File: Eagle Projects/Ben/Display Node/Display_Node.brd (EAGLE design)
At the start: 100 x 80 mm, 29 parts, among them Q1 16MHz, Q3 16MHz, Q4 16MHz, U1 ATMEGA328P_TQFP, U2 MCP2551

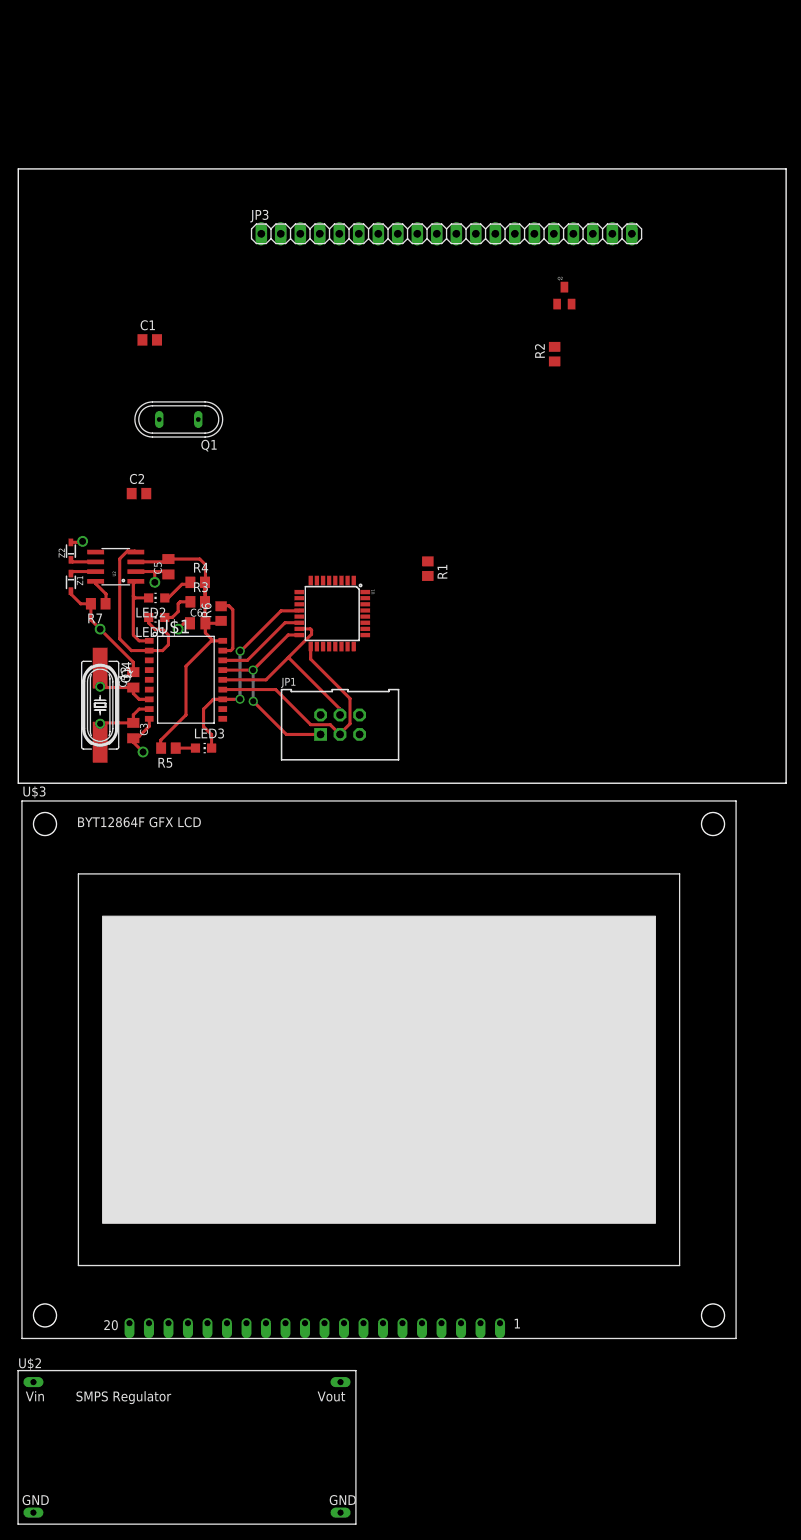
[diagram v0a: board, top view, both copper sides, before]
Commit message: Workin on stuff...
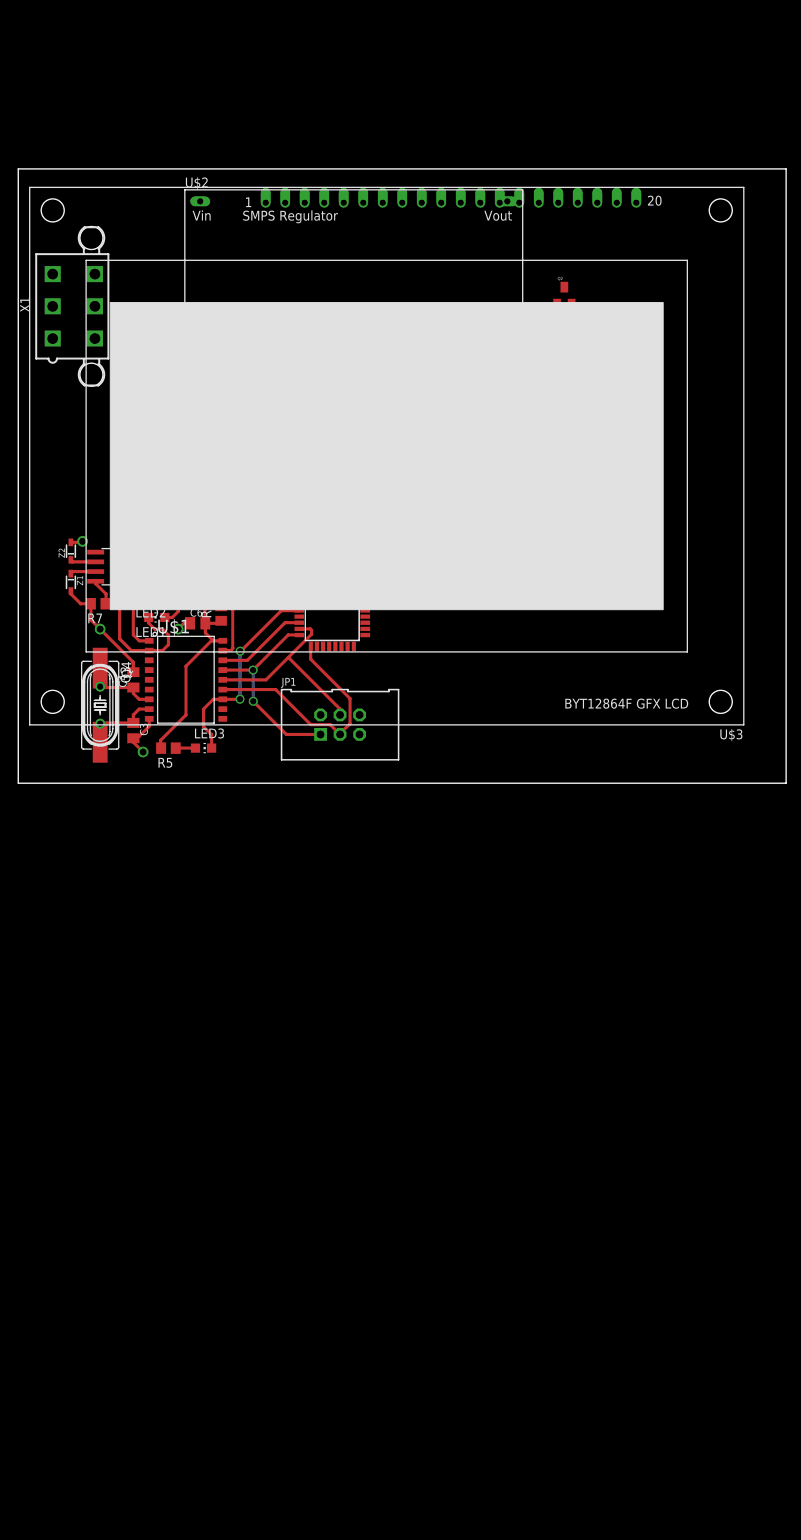
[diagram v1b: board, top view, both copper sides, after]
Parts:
- removed JP3: GFX_LCD, adafruit:1X20
- added X1, X2: 5566-6, con-molex:5566-6
- moved U$3 176.9 mm to (94.5, 77.6), turned to 180 degrees
- moved U$2 155.3 mm to (21.7, 57.3)
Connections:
- new net +12V: U$2.VIN, X1.1, X2.1
- new net LCD_RST: U$3.P$4
- new net N$14: X1.5, X2.5
- new net N$15: X1.6, X2.6
- net +5V: now also U$2.VOUT, U$3.P$19, U$3.P$2; no longer JP3.17, JP3.19, JP3.2
- net CANH: now also X1.3, X2.3
- net CANL: now also X1.4, X2.4
- net GND: now also U$2.GND, U$2.GND@, U$3.P$20, U$3.P$6, X1.2, X2.2; no longer JP3.1, JP3.15
- net LCD_CS: now also U$3.P$17; no longer JP3.4
- net MOSI: now also U$3.P$16; no longer JP3.5
- net N$4: now also U$3.P$1; no longer JP3.20
- net SCK: now also U$3.P$15; no longer JP3.6

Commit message: Almost lost some important stuff! managed to save it :D
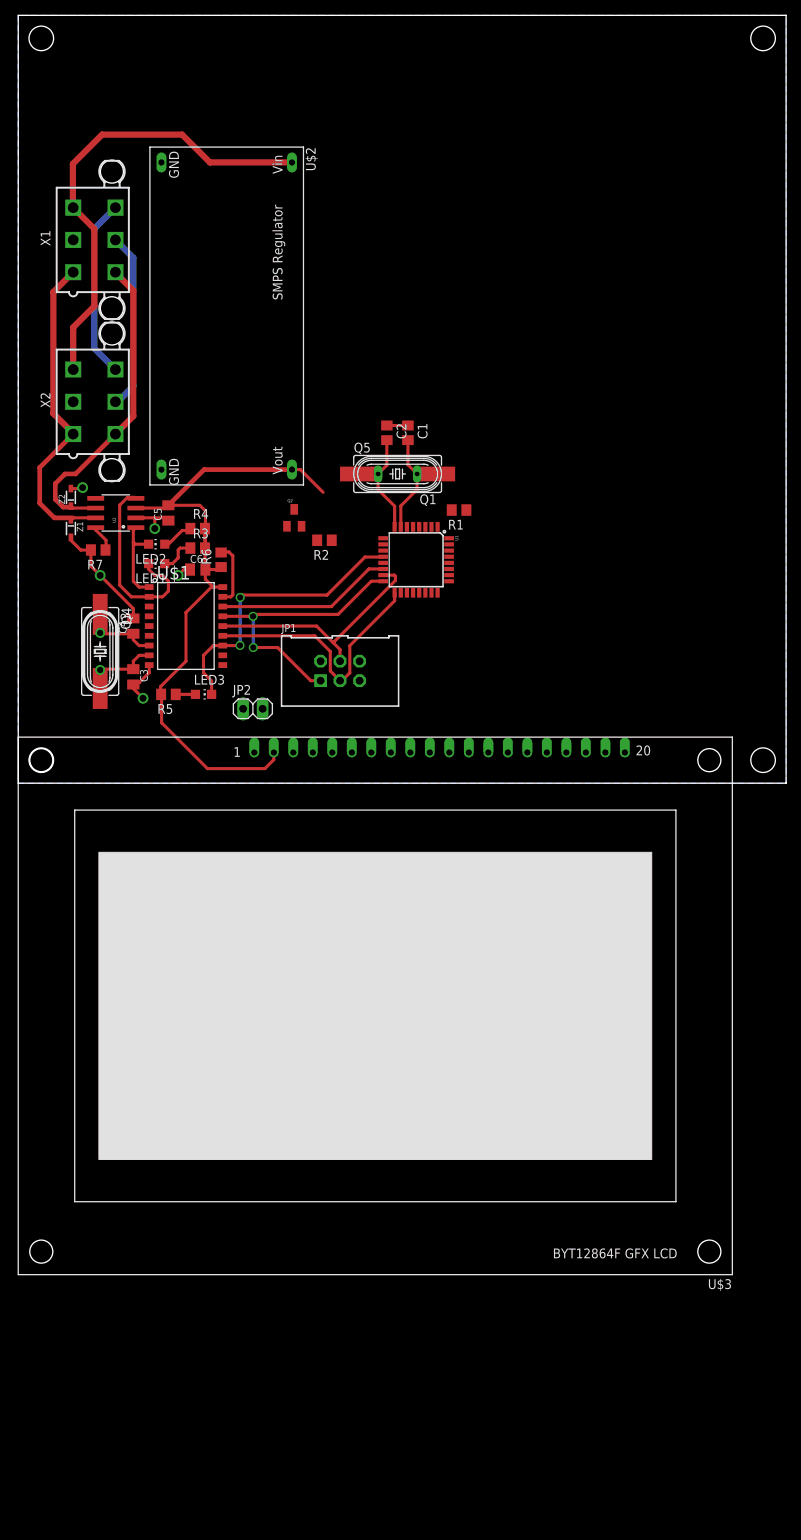
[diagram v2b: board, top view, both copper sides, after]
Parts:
- added JP2: (no value), pinhead:1X02
- added Q5: 16MHz, crystal:HC49UP
- moved U$3 71.6 mm to (93.0, 6.00)
- moved Q2 45.6 mm to (35.9, 34.6)
- moved R2 38.5 mm to (39.9, 31.6), turned to 180 degrees
- moved C1 35.7 mm to (50.7, 45.6), turned to 270 degrees
- moved C2 33.2 mm to (48.0, 45.6), turned to 270 degrees
- moved X2 32.4 mm to (9.91, 49.7)
- moved Q1 29.4 mm to (49.4, 40.3)
- moved U$2 26.0 mm to (17.1, 82.8), turned to 270 degrees
- moved U1 13.0 mm to (51.8, 29.1)
- moved X1 9.05 mm to (9.91, 70.8)
- moved R1 8.65 mm to (57.4, 35.6), turned to 180 degrees
- moved C5 7.00 mm to (19.6, 35.2)
- moved U2 7.00 mm to (12.7, 35.2)
- moved C3 7.00 mm to (15.0, 13.9)
- moved C4 7.00 mm to (15.0, 20.5)
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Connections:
- new net N$10: JP1.2, JP2.2
- net +12V: now also X1.3, X2.3; no longer X1.1, X2.1
- net +5V: now also JP2.1; no longer JP1.2
- net CANH: now also X1.1, X2.1; no longer X1.3, X2.3
- net N$1: now also Q5.2
- net N$2: now also Q5.1
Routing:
- net +12V: track 0.00 -> 60.7 mm
- net +5V: track 44.2 -> 90.3 mm
- net CANH: track 3.33 -> 42.5 mm
- net CANL: track 3.33 -> 41.4 mm
- net N$15: track 0.00 -> 23.4 mm
- net N$14: track 0.00 -> 23.2 mm
- net N$1: track 0.00 -> 12.7 mm
- net N$2: track 0.00 -> 12.7 mm
- net MISO: track 26.5 -> 37.6 mm
- net CANCS: track 12.0 -> 22.9 mm
- net CANINT: track 27.1 -> 38.1 mm
- net MOSI: track 26.5 -> 31.7 mm
- net GND: track 29.6 -> 32.3 mm
- net SCK: track 31.8 -> 33.8 mm
- added copper zone on layer 16, net GND
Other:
- board size 100 x 80 mm -> 100 x 100 mm
